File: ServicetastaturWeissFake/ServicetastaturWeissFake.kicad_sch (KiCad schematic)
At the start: 30 parts, among them J1 Automat, SW1 SW_Push, SW10 SW_Push, SW11 SW_Push, SW12 SW_Push, SW13 SW_Push, SW14 SW_Push, SW15 SW_Push, SW16 SW_Push, SW2 SW_Push, SW3 SW_Push, SW4 SW_Push, SW5 SW_Push, SW6 SW_Push, SW7 SW_Push, SW8 SW_Push, SW9 SW_Push, U1 LTC-4627JD, U2 LTC-4627JD, U3 74LS48, U4 74LS145

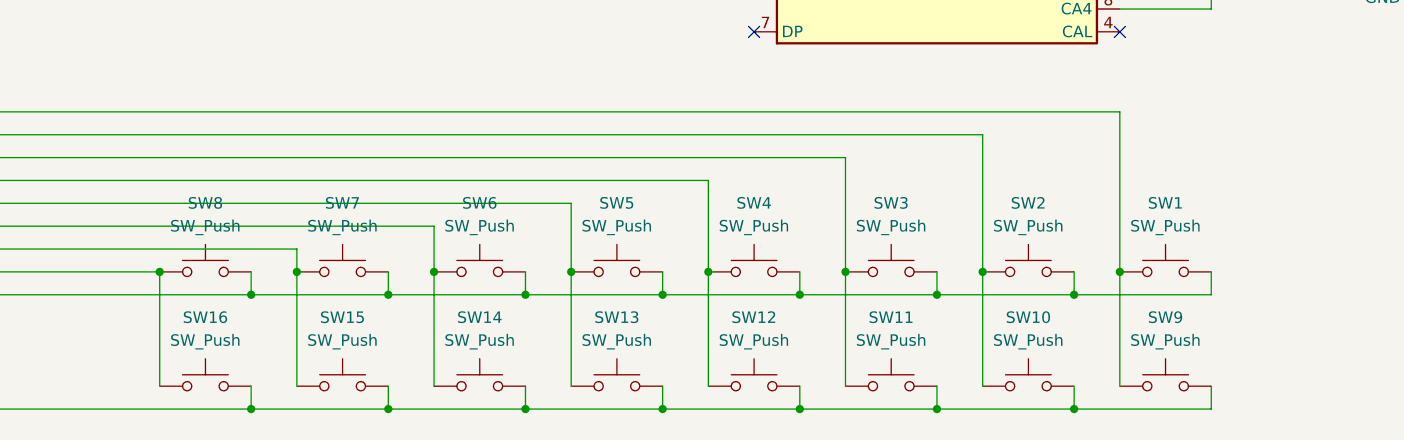
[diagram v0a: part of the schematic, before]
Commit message: beschriftung
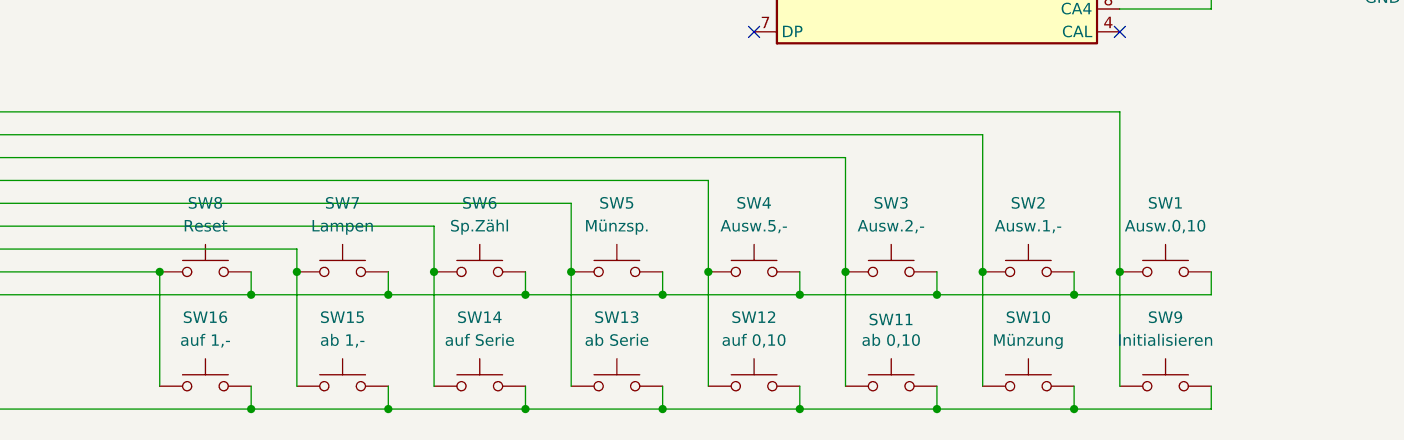
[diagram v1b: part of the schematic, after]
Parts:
- SW1: value SW_Push -> Ausw.0,10
- SW10: value SW_Push -> Münzung
- SW11: value SW_Push -> ab 0,10
- SW12: value SW_Push -> auf 0,10
- SW13: value SW_Push -> ab Serie
- SW14: value SW_Push -> auf Serie
- SW15: value SW_Push -> ab 1,-
- SW16: value SW_Push -> auf 1,-
- SW2: value SW_Push -> Ausw.1,-
- SW3: value SW_Push -> Ausw.2,-
- SW4: value SW_Push -> Ausw.5,-
- SW5: value SW_Push -> Münzsp.
- SW6: value SW_Push -> Sp.Zähl
- SW7: value SW_Push -> Lampen
- SW8: value SW_Push -> Reset
- SW9: value SW_Push -> Initialisieren
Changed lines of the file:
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@@
 			)
 		)
-		(property "Value" "SW_Push"
+		(property "Value" "ab Serie"
 			(at 147.32 147.32 0)
 			(effects
@@
 		(on_board yes)
 		(dnp no)
-		(fields_autoplaced yes)
 		(property "Reference" "SW11"
-			(at 177.8 144.78 0)
-			(effects
-				(font
-					(size 1.27 1.27)
-				)
-			)
-		)
-		(property "Value" "SW_Push"
+			(at 177.8 145.034 0)
+			(effects
+				(font
+					(size 1.27 1.27)
+				)
+			)
+		)
+		(property "Value" "ab 0,10"
 			(at 177.8 147.32 0)
 			(effects
@@
 			)
 		)
-		(property "Value" "SW_Push"
+		(property "Value" "Ausw.5,-"
 			(at 162.56 134.62 0)
 			(effects
@@
 		(on_board yes)
 		(dnp no)
-		(fields_autoplaced yes)
 		(property "Reference" "SW9"
 			(at 208.28 144.78 0)
@@
 			)
 		)
-		(property "Value" "SW_Push"
+		(property "Value" "Initialisieren"
 			(at 208.28 147.32 0)
 			(effects
@@
 			)
 		)
-		(property "Value" "SW_Push"
+		(property "Value" "Ausw.1,-"
 			(at 193.04 134.62 0)
 			(effects
@@
 			)
 		)
-		(property "Value" "SW_Push"
+		(property "Value" "Münzsp."
 			(at 147.32 134.62 0)
 			(effects
@@
 			)
 		)
-		(property "Value" "SW_Push"
+		(property "Value" "Sp.Zähl"
 			(at 132.08 134.62 0)
 			(effects
@@
 			)
 		)
-		(property "Value" "SW_Push"
+		(property "Value" "Ausw.2,-"
 			(at 177.8 134.62 0)
 			(effects
@@
 			)
 		)
-		(property "Value" "SW_Push"
+		(property "Value" "Lampen"
 			(at 116.84 134.62 0)
 			(effects
@@
 			)
 		)
-		(property "Value" "SW_Push"
+		(property "Value" "auf 0,10"
 			(at 162.56 147.32 0)
 			(effects
@@
 			)
 		)
-		(property "Value" "SW_Push"
+		(property "Value" "Münzung"
 			(at 193.04 147.32 0)
 			(effects
@@
 			)
 		)
-		(property "Value" "SW_Push"
+		(property "Value" "Reset"
 			(at 101.6 134.62 0)
 			(effects
@@
 			)
 		)
-		(property "Value" "SW_Push"
+		(property "Value" "auf Serie"
 			(at 132.08 147.32 0)
 			(effects
@@
 			)
 		)
-		(property "Value" "SW_Push"
+		(property "Value" "ab 1,-"
 			(at 116.84 147.32 0)
 			(effects
@@
 			)
 		)
-		(property "Value" "SW_Push"
+		(property "Value" "auf 1,-"
 			(at 101.6 147.32 0)
 			(effects
@@
 			)
 		)
-		(property "Value" "SW_Push"
+		(property "Value" "Ausw.0,10"
 			(at 208.28 134.62 0)
 			(effects

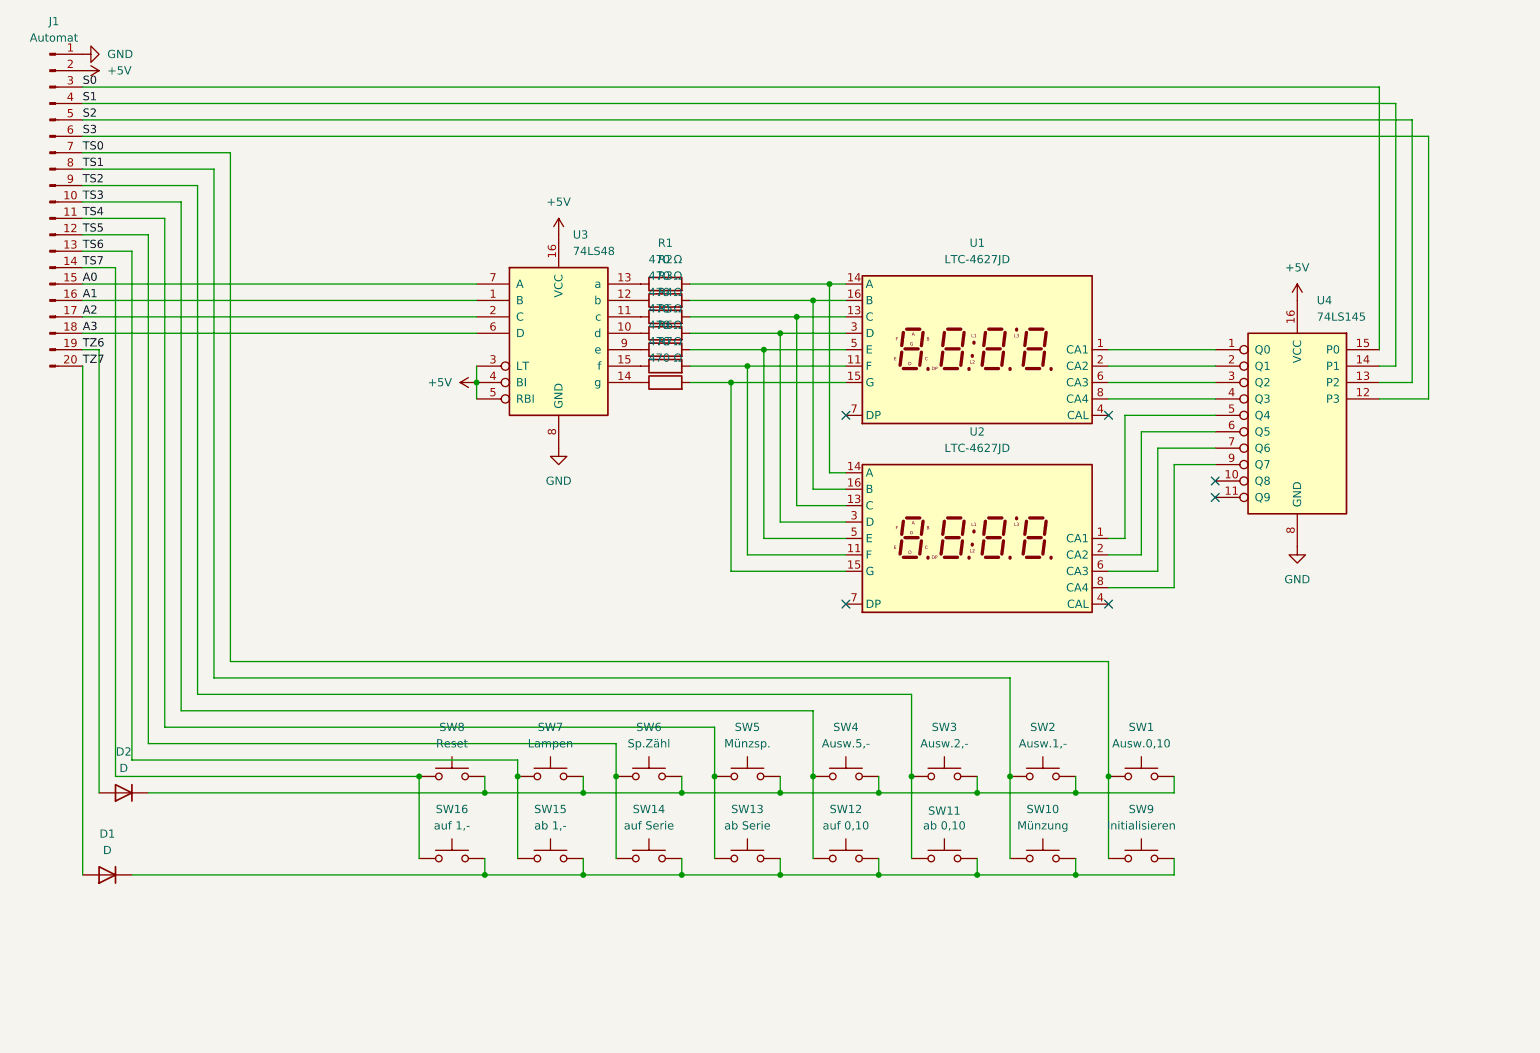
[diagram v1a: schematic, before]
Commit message: CC redesign
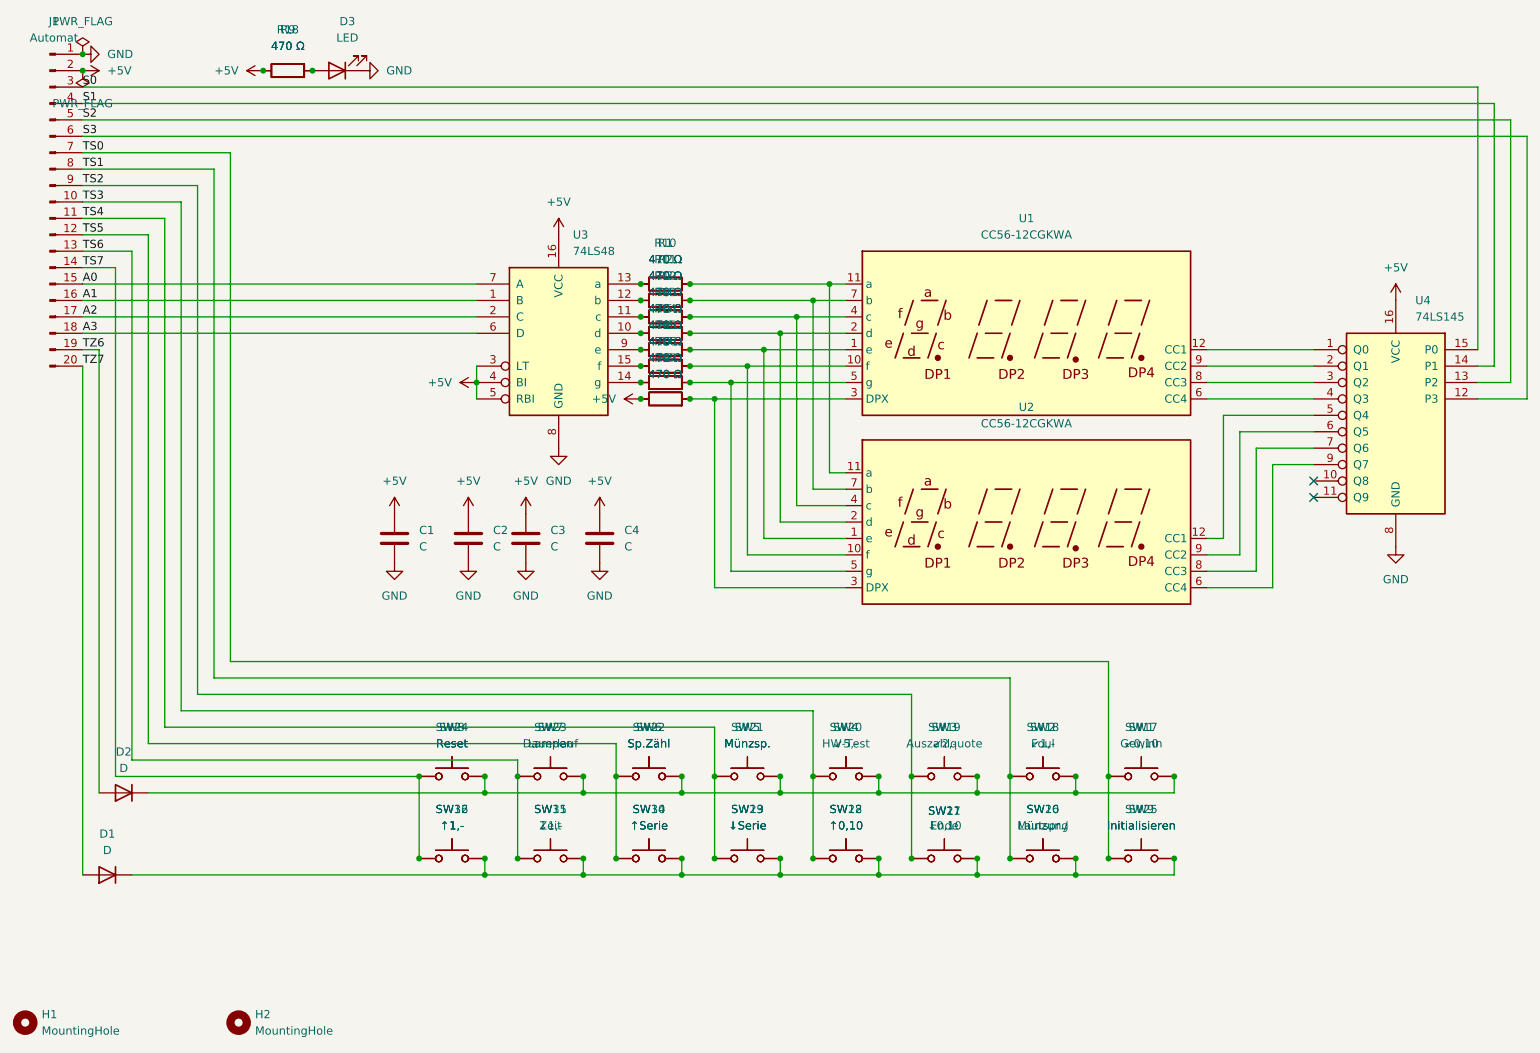
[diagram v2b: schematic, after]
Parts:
- removed U1, U2: LTC-4627JD, Display_7Segment:LTC-4627Jx, symbol Display_Character:LTC-4627JD
- added C1, C2: C, Capacitor_THT:C_Disc_D4.3mm_W1.9mm_P5.00mm, symbol Device:C
- added C3, C4: C, Capacitor_SMD:C_0805_2012Metric, symbol Device:C
- added D3: LED, LED_THT:LED_D5.0mm, symbol Device:LED
- added H1, H2: MountingHole, MountingHole:MountingHole_3.2mm_M3, symbol Mechanical:MountingHole
- added R10, R11, R12, R13, R14, R15, R16, R17, R18: 470 Ω, Resistor_SMD:R_0805_2012Metric, symbol Device:R
- added R8, R9: 470 Ω, Resistor_THT:R_Axial_DIN0207_L6.3mm_D2.5mm_P7.62mm_Horizontal, symbol Device:R
- added SW17: ↙0,10, Button_Switch_THT:SW_PUSH_6mm, symbol Switch:SW_Push
- added SW18: ↙1,-, Button_Switch_THT:SW_PUSH_6mm, symbol Switch:SW_Push
- added SW19: Auszahlquote, Button_Switch_THT:SW_PUSH_6mm, symbol Switch:SW_Push
- added SW20: ↙5,-, Button_Switch_THT:SW_PUSH_6mm, symbol Switch:SW_Push
- added SW21: Münzsp., Button_Switch_THT:SW_PUSH_6mm, symbol Switch:SW_Push
- added SW22: Sp.Zähl, Button_Switch_THT:SW_PUSH_6mm, symbol Switch:SW_Push
- added SW23: Lampen, Button_Switch_THT:SW_PUSH_6mm, symbol Switch:SW_Push
- added SW24: Reset, Button_Switch_THT:SW_PUSH_6mm, symbol Switch:SW_Push
- added SW25: Initialisieren, Button_Switch_THT:SW_PUSH_6mm, symbol Switch:SW_Push
- added SW26: Münzung, Button_Switch_THT:SW_PUSH_6mm, symbol Switch:SW_Push
- added SW27: Ende, Button_Switch_THT:SW_PUSH_6mm, symbol Switch:SW_Push
- added SW28: ↑0,10, Button_Switch_THT:SW_PUSH_6mm, symbol Switch:SW_Push
- added SW29: ↓Serie, Button_Switch_THT:SW_PUSH_6mm, symbol Switch:SW_Push
- added SW30: ↑Serie, Button_Switch_THT:SW_PUSH_6mm, symbol Switch:SW_Push
- added SW31: ↓1,-, Button_Switch_THT:SW_PUSH_6mm, symbol Switch:SW_Push
- added SW32: ↑1,-, Button_Switch_THT:SW_PUSH_6mm, symbol Switch:SW_Push
- added U1, U2: CC56-12CGKWA, Display_7Segment:CA56-12CGKWA, symbol Display_Character:CC56-12CGKWA
- R1, R2, R3, R4, R5, R6, R7: footprint Resistor_THT:R_Axial_DIN0207_L6.3mm_D2.5mm_P10.16mm_Horizontal -> Resistor_THT:R_Axial_DIN0207_L6.3mm_D2.5mm_P7.62mm_Horizontal
- SW1: value Ausw.0,10 -> Gewinn; footprint Button_Switch_THT:SW_PUSH_6mm -> Button_Switch_THT:SW_PUSH-12mm
- SW10: value Münzung -> Lautspr./; footprint Button_Switch_THT:SW_PUSH_6mm -> Button_Switch_THT:SW_PUSH-12mm
- SW11: value ab 0,10 -> ↓0,10; footprint Button_Switch_THT:SW_PUSH_6mm -> Button_Switch_THT:SW_PUSH-12mm
- SW12: value auf 0,10 -> ↑0,10; footprint Button_Switch_THT:SW_PUSH_6mm -> Button_Switch_THT:SW_PUSH-12mm
- SW13: value ab Serie -> ↓Serie; footprint Button_Switch_THT:SW_PUSH_6mm -> Button_Switch_THT:SW_PUSH-12mm
- SW14: value auf Serie -> ↑Serie; footprint Button_Switch_THT:SW_PUSH_6mm -> Button_Switch_THT:SW_PUSH-12mm
- SW15: value ab 1,- -> Zeit; footprint Button_Switch_THT:SW_PUSH_6mm -> Button_Switch_THT:SW_PUSH-12mm
- SW16: value auf 1,- -> ↑1,-; footprint Button_Switch_THT:SW_PUSH_6mm -> Button_Switch_THT:SW_PUSH-12mm
- SW2: value Ausw.1,- -> Foul; footprint Button_Switch_THT:SW_PUSH_6mm -> Button_Switch_THT:SW_PUSH-12mm
- SW3: value Ausw.2,- -> ↙2,-; footprint Button_Switch_THT:SW_PUSH_6mm -> Button_Switch_THT:SW_PUSH-12mm
- SW4: value Ausw.5,- -> HW-Test; footprint Button_Switch_THT:SW_PUSH_6mm -> Button_Switch_THT:SW_PUSH-12mm
- SW5, SW6, SW8, SW9: footprint Button_Switch_THT:SW_PUSH_6mm -> Button_Switch_THT:SW_PUSH-12mm
- SW7: value Lampen -> Dauerlauf; footprint Button_Switch_THT:SW_PUSH_6mm -> Button_Switch_THT:SW_PUSH-12mm
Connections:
- net +5V: now also C1.1, C2.1, C3.1, C4.1, R17.1, R18.1, R8.1, R9.1
- net GND: now also C1.2, C2.2, C3.2, C4.2, D3.1 (K)
- net TS0: now also SW17.2, SW25.2
- net TS1: now also SW18.2, SW26.2
- net TS2: now also SW19.2, SW27.2
- net TS3: now also SW20.2, SW28.2
- net TS4: now also SW21.2, SW29.2
- net TS5: now also SW22.2, SW30.2
- net TS6: now also SW23.2, SW31.2
- net TS7: now also SW24.2, SW32.2
- net at D1.1 (K), SW10.1, SW11.1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: now also SW25.1, SW26.1, SW27.1, SW28.1, SW29.1, SW30.1, SW31.1, SW32.1
- net at R2.1, U3.12 (b): now also R11.1
- net at R2.2: now also R11.2, U1.7 (b), U2.7 (b)
- net at R4.1, U3.10 (d): now also R13.1
- net at R4.2: now also R13.2, U1.2 (d), U2.2 (d)
- net at D2.1 (K), SW1.1, SW2.1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: now also SW17.1, SW18.1, SW19.1, SW20.1, SW21.1, SW22.1, SW23.1, SW24.1
- net at R3.1, U3.11 (c): now also R12.1
- net at R3.2: now also R12.2, U1.4 (c), U2.4 (c)
- net at R5.1, U3.9 (e): now also R14.1
- net at R5.2: now also R14.2, U1.1 (e), U2.1 (e)
- net at U4.1 (Q0): now also U1.12 (CC1)
- net at U4.2 (Q1): now also U1.9 (CC2)
- net at U4.3 (Q2): now also U1.8 (CC3)
- net at U4.4 (Q3): now also U1.6 (CC4)
- net at U4.5 (Q4): now also U2.12 (CC1)
- net at U4.6 (Q5): now also U2.9 (CC2)
- net at U4.7 (Q6): now also U2.8 (CC3)
- net at U4.9 (Q7): now also U2.6 (CC4)
- net at R6.2: now also R15.2, U1.10 (f), U2.10 (f)
- net at R1.2: now also R10.2, U1.11 (a), U2.11 (a)
- net at R7.2: now also R16.2, U1.5 (g), U2.5 (g)
- net at R6.1, U3.15 (f): now also R15.1
- net at R1.1, U3.13 (a): now also R10.1
- net at R7.1, U3.14 (g): now also R16.1
- new net: R17.2, R8.2, U1.3 (DPX), U2.3 (DPX)
- new net: D3.2 (A), R18.2, R9.2
- no-connect marks 6 -> 2
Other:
- moved on the sheet: U4
